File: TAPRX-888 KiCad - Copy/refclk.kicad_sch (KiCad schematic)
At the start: 57 parts, among them J10 U.FL-R, Q1 PMOS Si2343DS, Q2 MMBT3904, Q3 PMOS Si2343DS, U14 LP5907MFX-3.3, U16 TLV3501, U18 NC7SV157, U19 74LVC2G14, U20 Si5351A, U21 NC7SV157, U22 SN65LVDS1, X1 TCXO-27M

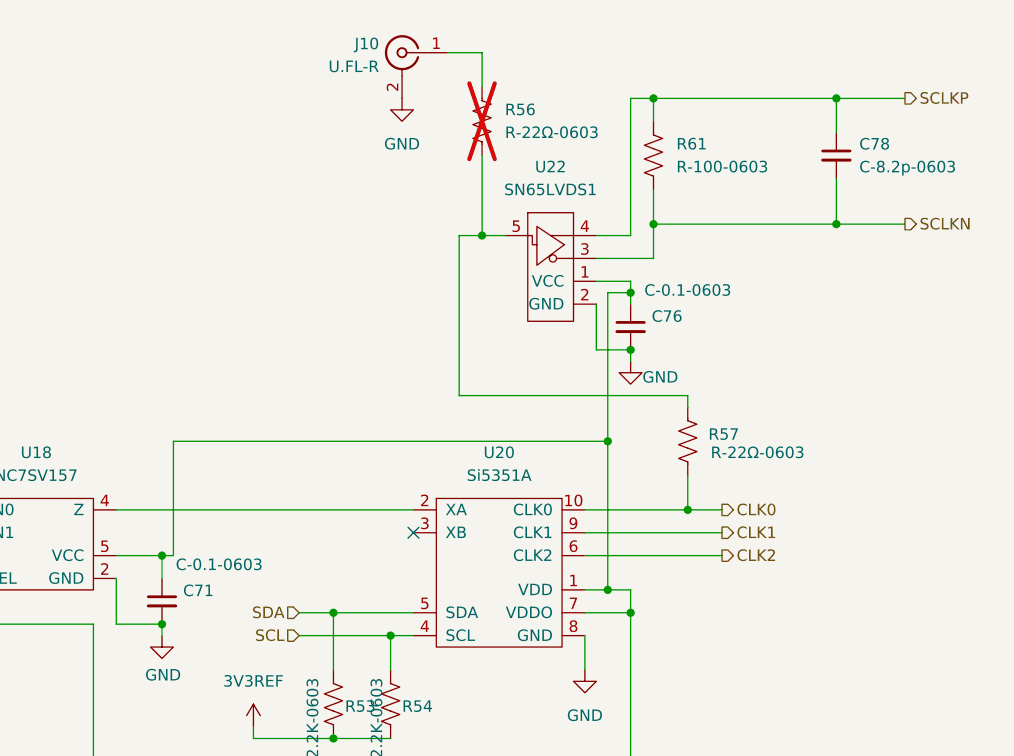
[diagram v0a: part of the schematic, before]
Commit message: proper update
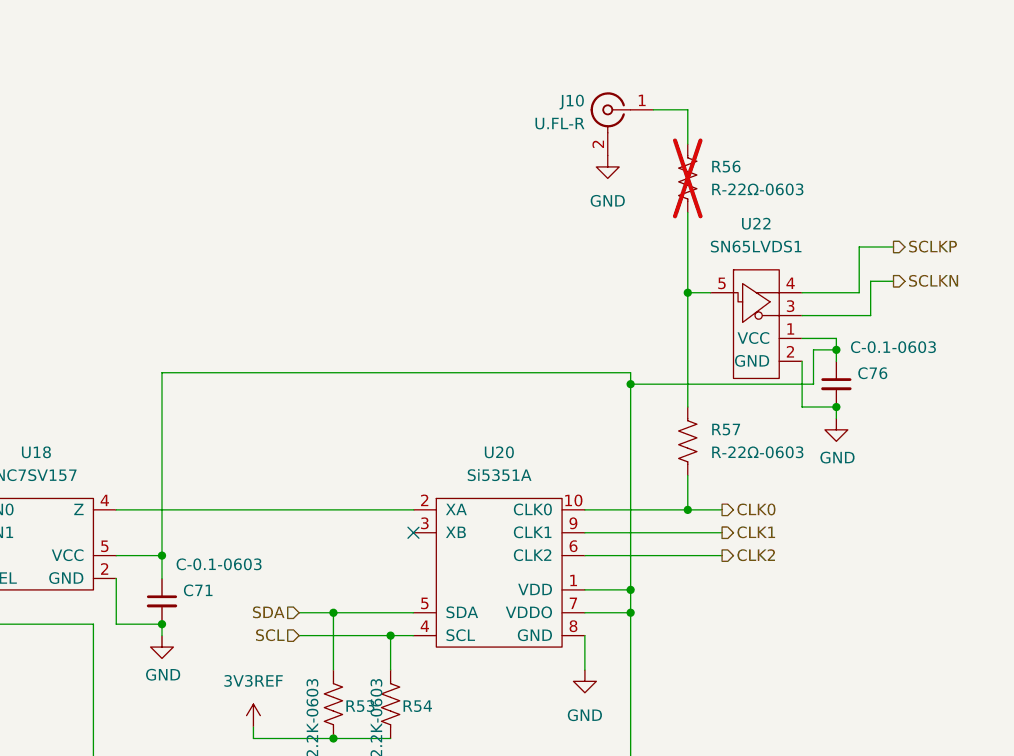
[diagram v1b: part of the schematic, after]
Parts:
- removed C78: C-8.2p-0603, TIS_Footprints:PAD_0603, symbol capacitors:C-8.2p-0603
- removed R61: R-100-0603, TIS_Footprints:PAD_0603, symbol resistors:R-100-0603
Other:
- moved on the sheet: C76, J10, R56, U22
